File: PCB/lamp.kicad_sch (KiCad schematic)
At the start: 3 parts, among them Q1 NMOS, U1 XIAO ESP32C3

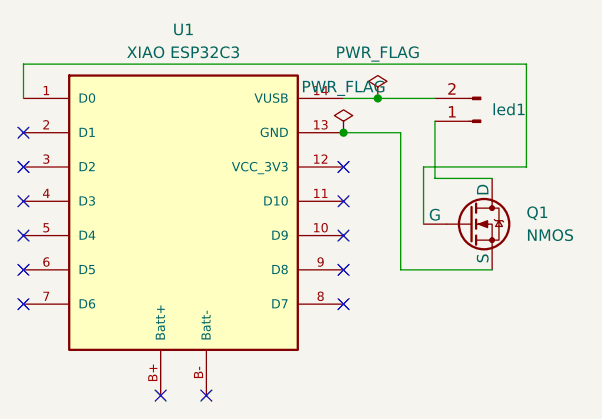
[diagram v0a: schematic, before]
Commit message: Add files via upload
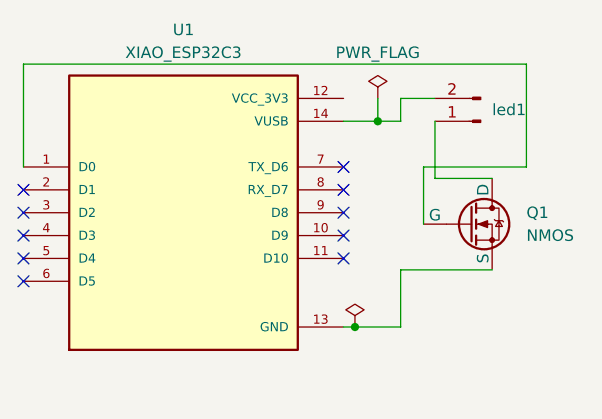
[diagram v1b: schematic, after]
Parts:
- removed U1: XIAO ESP32C3, RF:xiao, symbol xiao_esp32c3:XIAO ESP32C3
- added U1: XIAO_ESP32C3, RF:xiao, symbol xiao:XIAO_ESP32C3
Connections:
- net at led1.2 (Pin_2): now also U1.14 (VUSB)
- net at Q1.2 (G): now also U1.1 (D0)
- net at Q1.3 (S): now also U1.13 (GND)
- no-connect marks 13 -> 10
